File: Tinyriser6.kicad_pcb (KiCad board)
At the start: 4 copper layers, 113.2 x 23.5 mm, 25 parts, among them J1 Bus_M.2_Socket_M, J2 Bus_PCI_Express_x16, J3 Conn_02x04_Odd_Even, J6 USB_A, J7 Conn_02x10_Odd_Even, M1 Fan_4pin

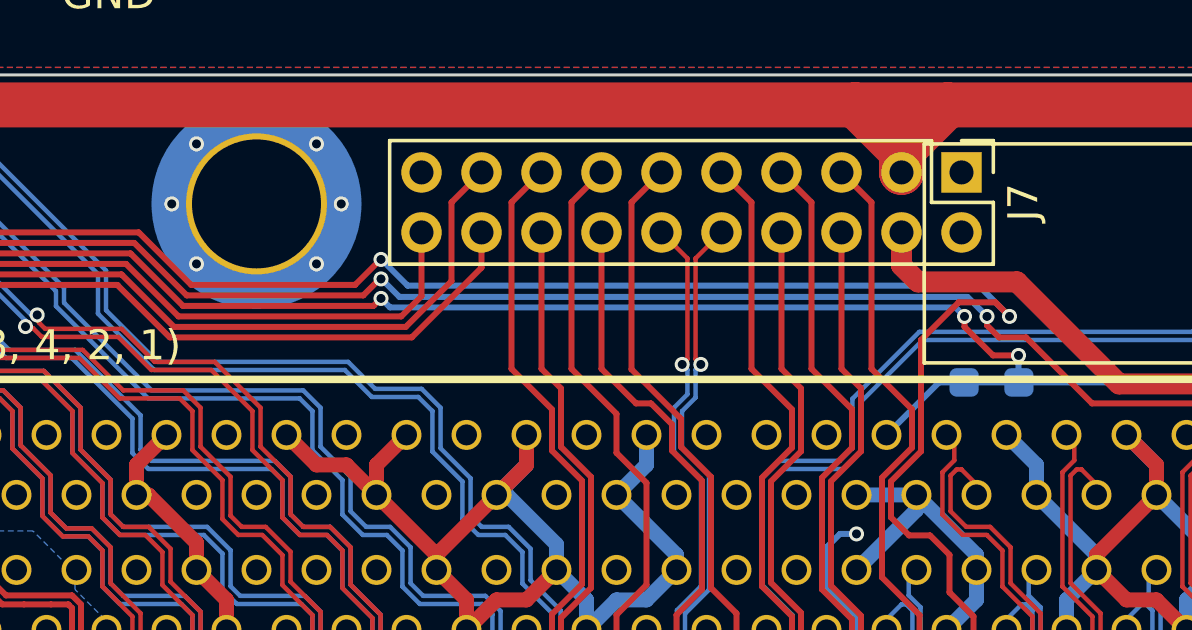
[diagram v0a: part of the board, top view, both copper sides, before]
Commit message: fixed some layer conflicts
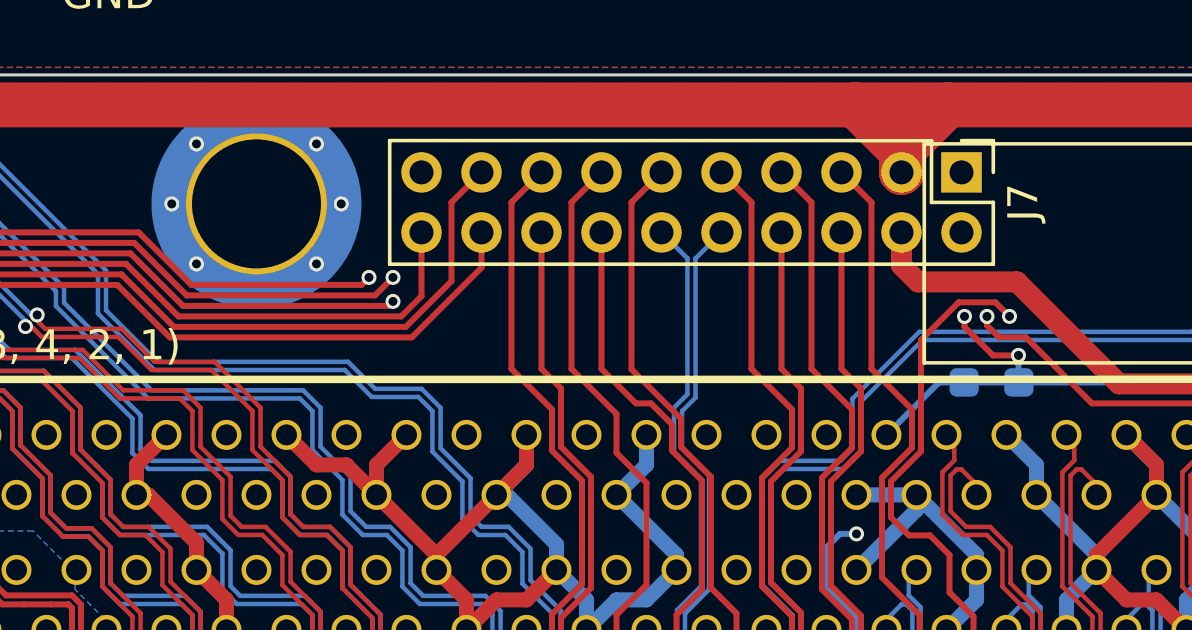
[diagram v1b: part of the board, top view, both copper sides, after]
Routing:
- net PERST#: track 159.0 -> 172.1 mm
- net PCIe_CPU_CLKREQ#: track 119.9 -> 132.7 mm
- net PCIe_PCH_CLKREQ#: track 84.6 -> 96.9 mm
- net PCIe_CPU_REFCLK11+: track 17.5 -> 17.4 mm, vias 1 -> 0
- net PCIe_CPU_REFCLK11-: track 17.5 -> 17.4 mm, vias 1 -> 0
